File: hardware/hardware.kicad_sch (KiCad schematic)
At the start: 25 parts, among them J1 USB_B_Micro, J2 Conn_Coaxial, Q1 BSS138, Q2 BSS138, U1 ESP32-WROOM-32, U2 AMS1117-3.3, U4 CH340C, U5 RFM95W-868S2

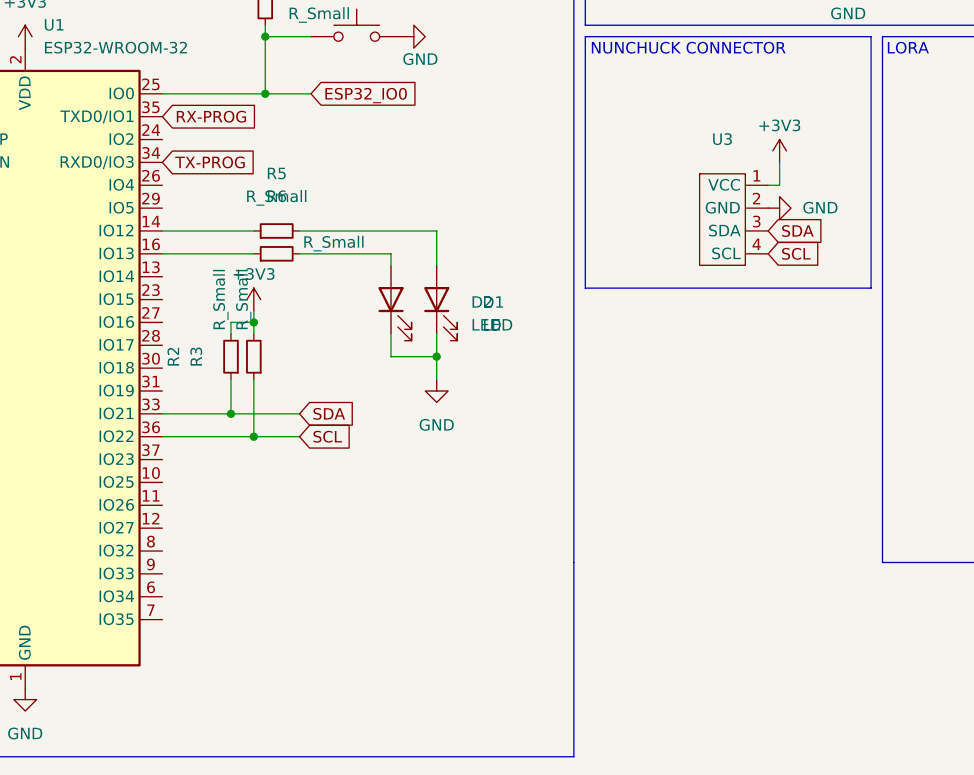
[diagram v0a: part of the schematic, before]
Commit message: lora wiring + pcb wiring
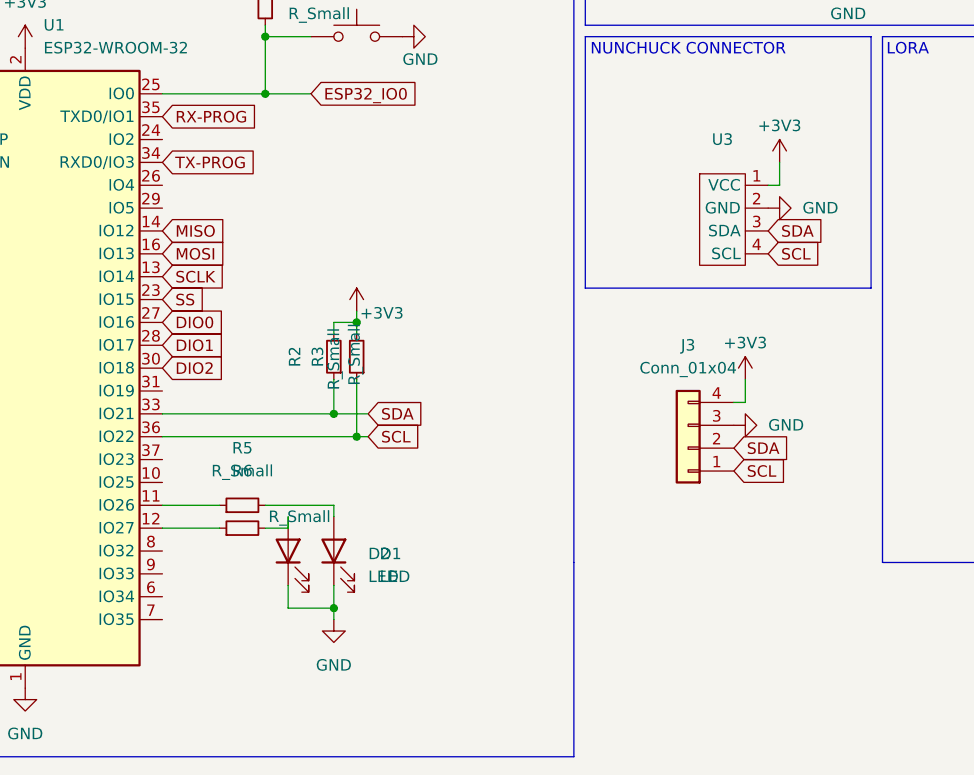
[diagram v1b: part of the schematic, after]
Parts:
- added J3: Conn_01x04, Connector_PinHeader_2.54mm:PinHeader_1x04_P2.54mm_Vertical, symbol Connector_Generic:Conn_01x04
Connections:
- net +3V3: now also J3.4 (Pin_4)
- net DIO0: now also U1.27 (IO16)
- net DIO1: now also U1.28 (IO17)
- net DIO2: now also U1.30 (IO18)
- net GND: now also J3.3 (Pin_3)
- net MISO: now also U1.14 (IO12)
- net MOSI: now also U1.16 (IO13)
- net SCL: now also J3.1 (Pin_1)
- net SCLK: now also U1.13 (IO14)
- net SDA: now also J3.2 (Pin_2)
- net SS: now also U1.23 (IO15)
- net at U1.11 (IO26): now also R5.1
- net at U1.12 (IO27): now also R6.1
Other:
- moved on the sheet: D1, D2, R2, R3, R5, R6
